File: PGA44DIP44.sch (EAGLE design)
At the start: 2 parts

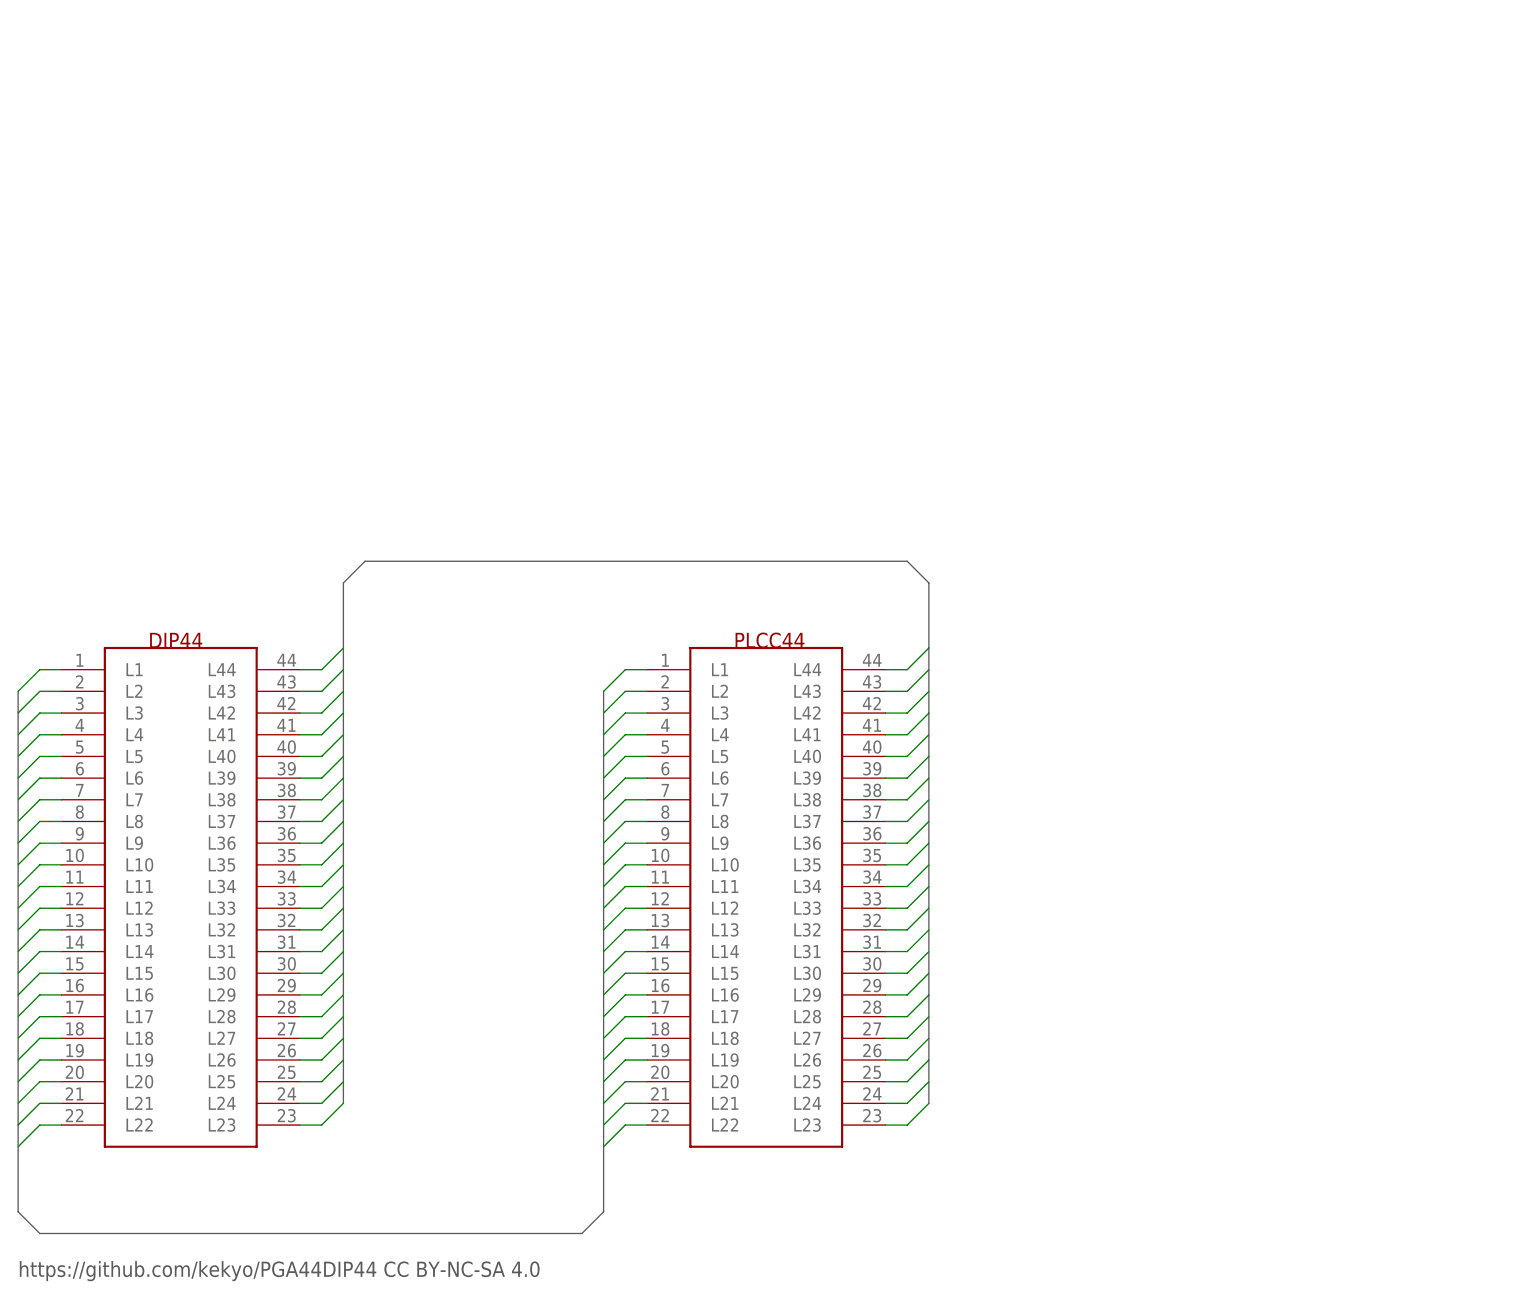
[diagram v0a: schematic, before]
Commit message: Artwork predesigning (WIP)
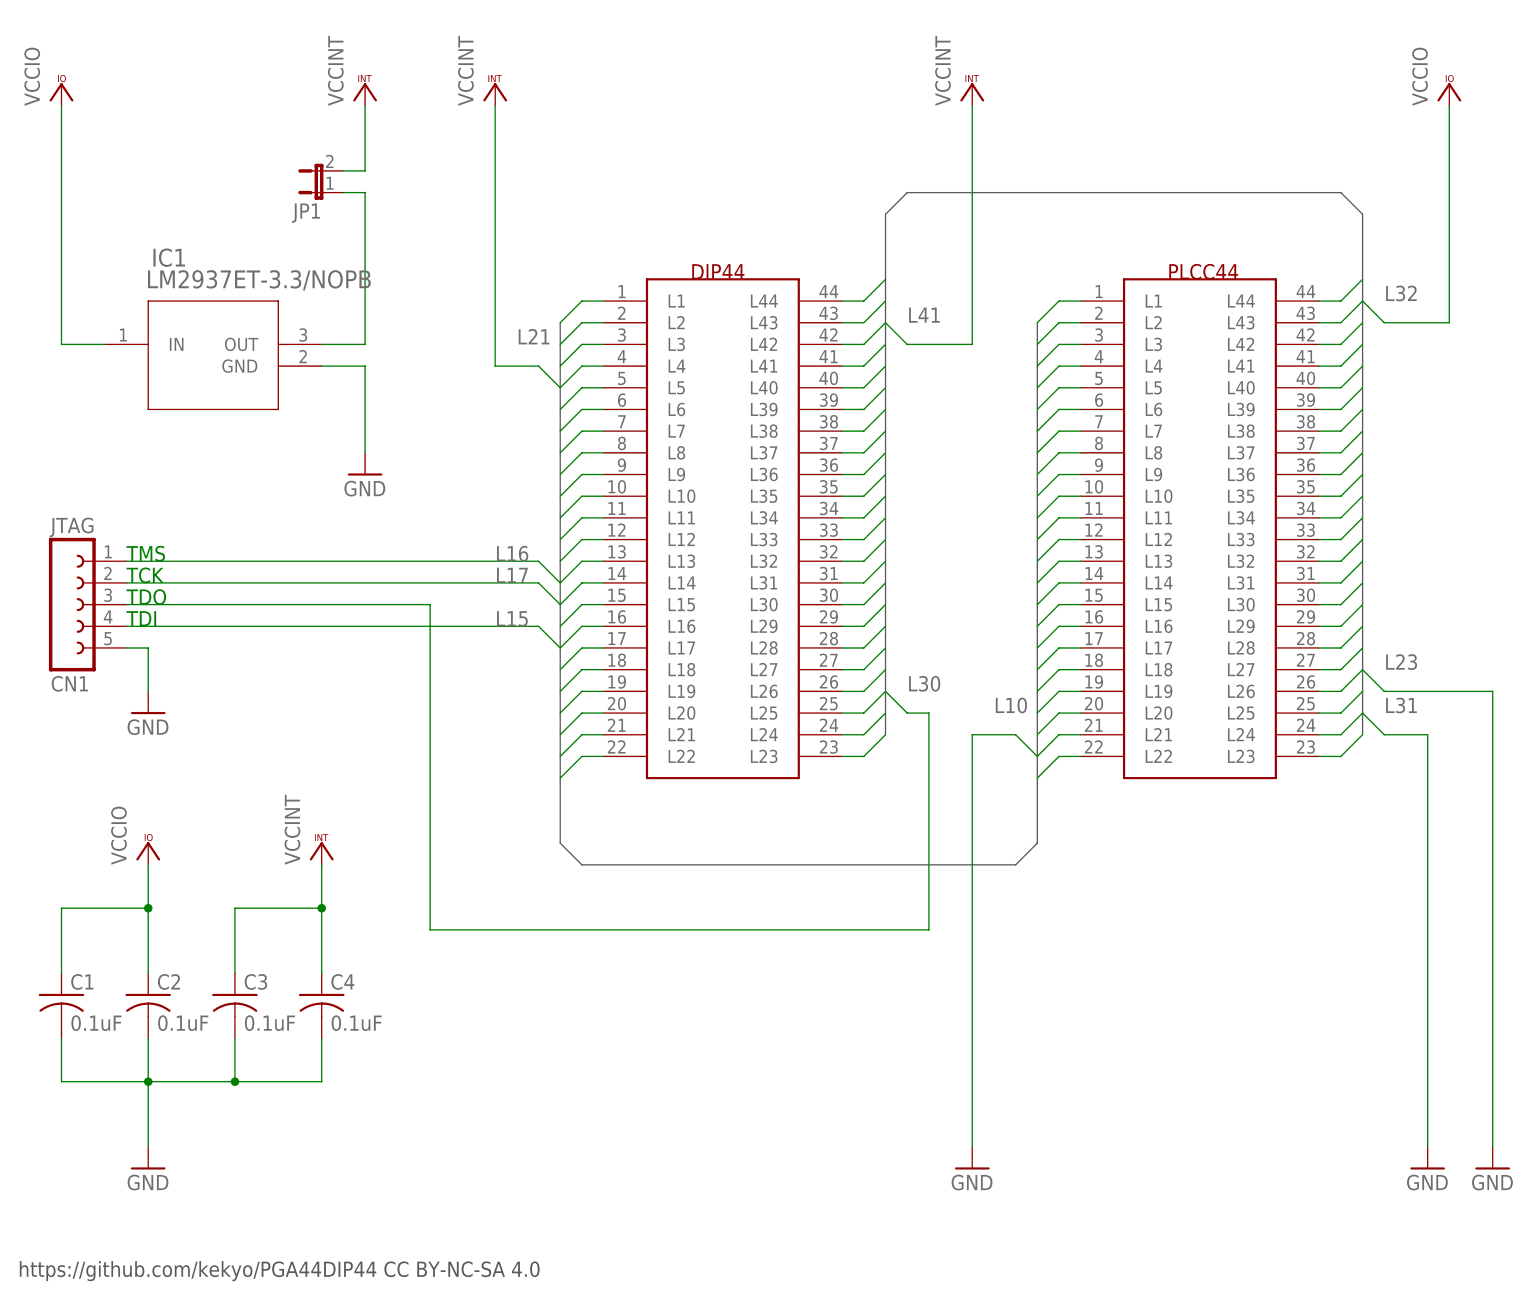
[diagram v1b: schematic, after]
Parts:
- added C1, C2, C3, C4: 0.1uF, rcl:C-US050-024X044
- added CN1: JTAG, con-lsta:FE05-1
- added IC1: LM2937ET-3.3/NOPB, PGA44DIP44:LM2937ET-3.3/NOPB
- added JP1: (no value), PGA44DIP44:JP1E
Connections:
- new net GND: C1.2, C2.2, C3.2, C4.2, CN1.5, IC1.GND
- new net N$1: IC1.OUT, JP1.1
- new net VCCINT: C3.1, C4.1, JP1.2
- new net VCCIO: C1.1, C2.1, IC1.IN
- net L15: now also CN1.4
- net L16: now also CN1.1
- net L17: now also CN1.2
- net L30: now also CN1.3
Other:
- note added: "TCK"
- note added: "TDI"
- note added: "TDO"
- note added: "TMS"
- moved on the sheet: DIP44, PLCC44
